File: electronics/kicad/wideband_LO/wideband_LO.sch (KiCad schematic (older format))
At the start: 25 parts, among them U1 BFP620

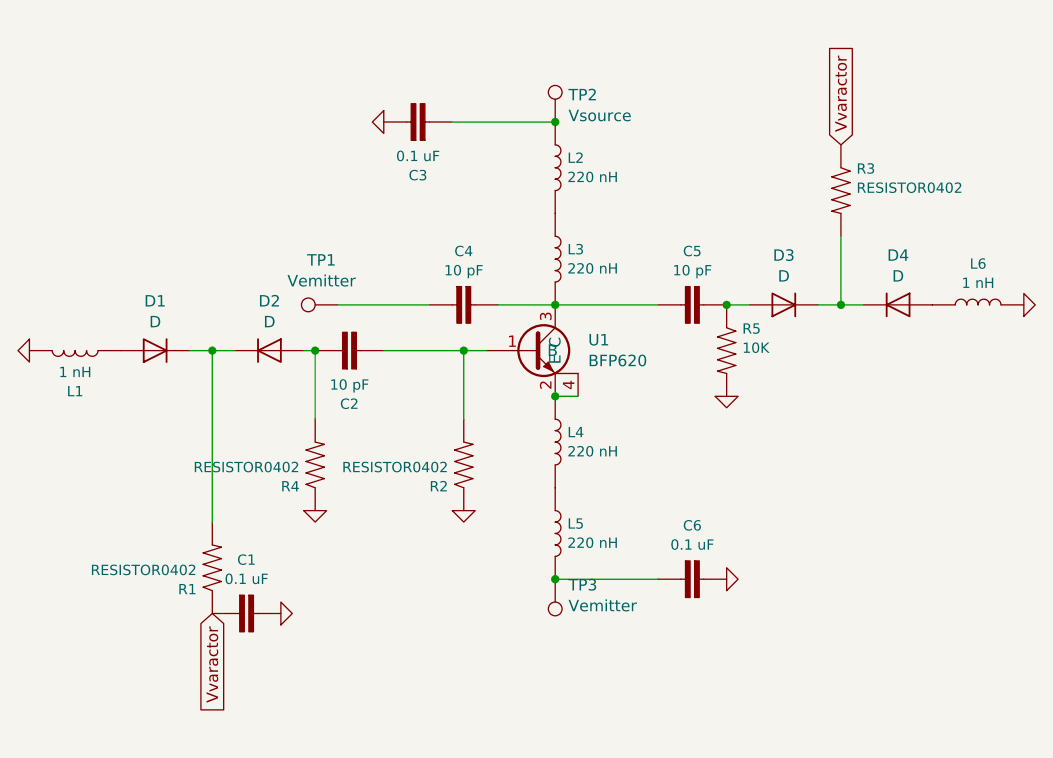
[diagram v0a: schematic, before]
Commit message: further fdtd
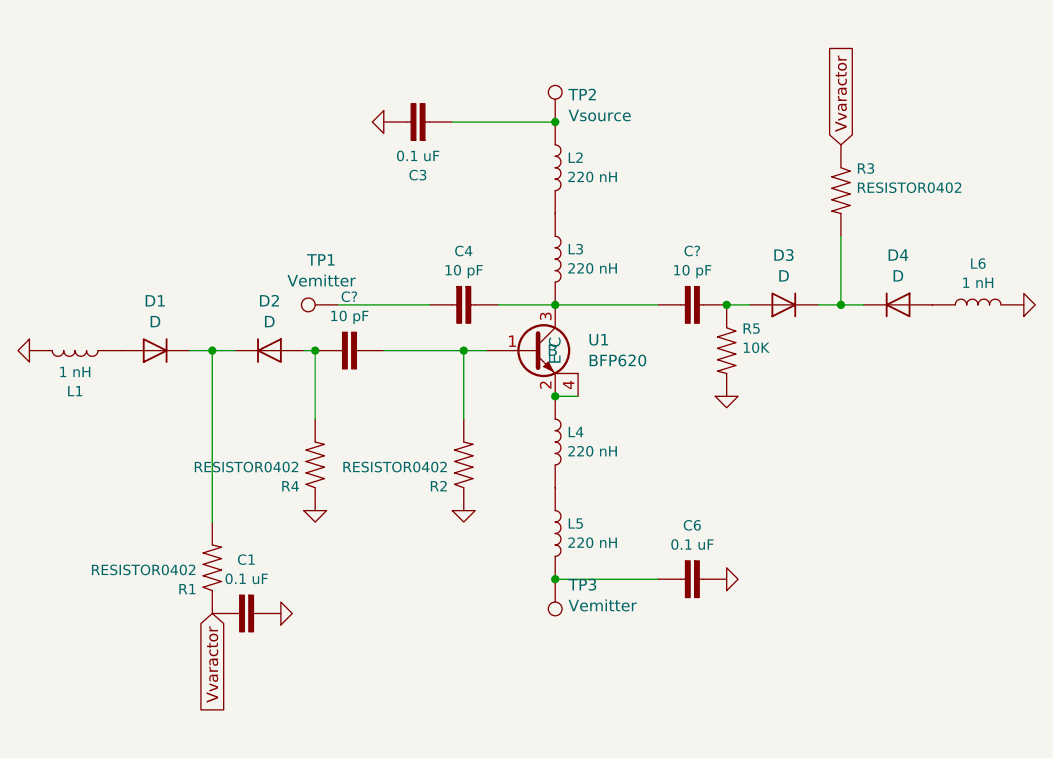
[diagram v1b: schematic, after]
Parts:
- removed C2, C5: 10 pF, 0402, symbol SparkFun-Capacitors:6PF-0402-50V-0.5%
- added C? (x2): 10 pF, 0402, symbol SparkFun-Capacitors:6PF-0402-50V-0.5%
- C4: Spice_Lib_File (none) -> /home/arthurdent/Projects/covidinator/electronics/models/10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; Spice_Model (none) -> 10pf0402; Spice_Netlist_Enabled (none) -> Y; Spice_Primitive (none) -> X
- D2: Spice_Lib_File (none) -> /home/arthurdent/Projects/covidinator/electronics/models/SM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; Spice_Model (none) -> SMV2019079LF; Spice_Netlist_Enabled (none) -> Y; Spice_Primitive (none) -> X
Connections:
- net at R2.2, U1.1 (B): now also C?.1
- net at C4.1, L3.2, U1.3 (C): now also C?.2
- net at D3.2 (A), R5.1: now also C?.1
- net at D2.2 (A), R4.2: now also C?.2
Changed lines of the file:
@@
 Wire Wire Line
 	3500 3050 3950 3050
-$Comp
-L SparkFun-Capacitors:6PF-0402-50V-0.5% C5
-U 1 1 5EE0CC0E
-P 4050 3050
-F 0 "C5" V 3816 3100 45  0000 C CNN
-F 1 "10 pF" V 3900 3100 45  0000 C CNN
-F 2 "0402" H 4050 3300 20  0001 C CNN
-F 3 "" H 4050 3050 50  0001 C CNN
-F 4 "" H 4158 3016 60  0000 L CNN "Field4"
-	1    4050 3050
-	0    1    1    0
-$EndComp
 Wire Wire Line
 	4850 3050 4750 3050
@@
 Wire Wire Line
 	3200 3250 3100 3250
-$Comp
-L SparkFun-Capacitors:6PF-0402-50V-0.5% C2
-U 1 1 5EE21BEE
-P 2650 3250
-F 0 "C2" V 2416 3300 45  0000 C CNN
-F 1 "10 pF" V 2500 3300 45  0000 C CNN
-F 2 "0402" H 2650 3500 20  0001 C CNN
-F 3 "" H 2650 3250 50  0001 C CNN
-F 4 "" H 2758 3216 60  0000 L CNN "Field4"
-	1    2650 3250
-	0    -1   -1   0
-$EndComp
 Wire Wire Line
 	1900 3250 2000 3250
-$Comp
-L SparkFun-Coils:INDUCTOR-0402-3.9NH L1
-U 1 1 5EE21BFD
-P 1400 3250
-F 0 "L1" V 1579 3250 45  0000 C CNN
-F 1 "1 nH" V 1495 3250 45  0000 C CNN
-F 2 "0402" H 1400 3500 20  0001 C CNN
-F 3 "" H 1400 3250 50  0001 C CNN
-F 4 "" H 1452 3166 60  0000 L CNN "Field4"
-	1    1400 3250
-	0    1    1    0
-$EndComp
-$Comp
-L power:GND #PWR0102
-U 1 1 5EE21C04
-P 1200 3250
-F 0 "#PWR0102" H 1200 3250 30  0001 C CNN
-F 1 "GND" H 1200 3180 30  0001 C CNN
-F 2 "" H 1200 3250 50  0001 C CNN
-F 3 "" H 1200 3250 50  0001 C CNN
-	1    1200 3250
-	0    1    1    0
-$EndComp
 $Comp
 L SparkFun-Resistors:RESISTOR0402 R1
@@
 F 3 "" H 3050 3050 50  0001 C CNN
 F 4 "" H 3158 3016 60  0000 L CNN "Field4"
+F 5 "X" H 3050 3050 50  0001 C CNN "Spice_Primitive"
+F 6 "10pf0402" H 3050 3050 50  0001 C CNN "Spice_Model"
+F 7 "Y" H 3050 3050 50  0001 C CNN "Spice_Netlist_Enabled"
+F 8 "/home/arthurdent/Projects/covidinator/electronics/models/10pf0402.lib" H 3050 3050 50  0001 C CNN "Spice_Lib_File"
 	1    3050 3050
 	0    1    1    0
@@
 F 2 "Diode_SMD:D_SOD-523" H 2250 3250 50  0001 C CNN
 F 3 "~" H 2250 3250 50  0001 C CNN
+F 4 "X" H 2250 3250 50  0001 C CNN "Spice_Primitive"
+F 5 "SMV2019079LF" H 2250 3250 50  0001 C CNN "Spice_Model"
+F 6 "Y" H 2250 3250 50  0001 C CNN "Spice_Netlist_Enabled"
+F 7 "/home/arthurdent/Projects/covidinator/electronics/models/SMV2019079LF.lib" H 2250 3250 50  0001 C CNN "Spice_Lib_File"
 	1    2250 3250
 	1    0    0    -1
@@
 Wire Wire Line
 	2400 3250 2450 3250
-Connection ~ 2450 3250
 $Comp
 L Device:D D3
@@
 Wire Wire Line
 	4350 3050 4250 3050
+$Comp
+L power:GND #PWR0102
+U 1 1 5EE21C04
+P 1200 3250
+F 0 "#PWR0102" H 1200 3250 30  0001 C CNN
+F 1 "GND" H 1200 3180 30  0001 C CNN
+F 2 "" H 1200 3250 50  0001 C CNN
+F 3 "" H 1200 3250 50  0001 C CNN
+	1    1200 3250
+	0    1    1    0
+$EndComp
+$Comp
+L SparkFun-Coils:INDUCTOR-0402-3.9NH L1
+U 1 1 5EE21BFD
+P 1400 3250
+F 0 "L1" V 1579 3250 45  0000 C CNN
+F 1 "1 nH" V 1495 3250 45  0000 C CNN
+F 2 "0402" H 1400 3500 20  0001 C CNN
+F 3 "" H 1400 3250 50  0001 C CNN
+F 4 "" H 1452 3166 60  0000 L CNN "Field4"
+	1    1400 3250
+	0    1    1    0
+$EndComp
+$Comp
+L SparkFun-Capacitors:6PF-0402-50V-0.5% C?
+U 1 1 5EEB34DA
+P 4050 3050
+F 0 "C?" V 3816 3100 45  0000 C CNN
+F 1 "10 pF" V 3900 3100 45  0000 C CNN
+F 2 "0402" H 4050 3300 20  0001 C CNN
+F 3 "" H 4050 3050 50  0001 C CNN
+F 4 "" H 4158 3016 60  0000 L CNN "Field4"
+F 5 "X" H 4050 3050 50  0001 C CNN "Spice_Primitive"
+F 6 "10pf0402" H 4050 3050 50  0001 C CNN "Spice_Model"
+F 7 "Y" H 4050 3050 50  0001 C CNN "Spice_Netlist_Enabled"
+F 8 "/home/arthurdent/Projects/covidinator/electronics/models/10pf0402.lib" H 4050 3050 50  0001 C CNN "Spice_Lib_File"
+	1    4050 3050
+	0    1    1    0
+$EndComp
 Connection ~ 4250 3050
+$Comp
+L SparkFun-Capacitors:6PF-0402-50V-0.5% C?
+U 1 1 5EEB3D3A
+P 2550 3250
+F 0 "C?" V 2316 3300 45  0000 C CNN
+F 1 "10 pF" V 2400 3300 45  0000 C CNN
+F 2 "0402" H 2550 3500 20  0001 C CNN
+F 3 "" H 2550 3250 50  0001 C CNN
+F 4 "" H 2658 3216 60  0000 L CNN "Field4"
+F 5 "X" H 2550 3250 50  0001 C CNN "Spice_Primitive"
+F 6 "10pf0402" H 2550 3250 50  0001 C CNN "Spice_Model"
+F 7 "Y" H 2550 3250 50  0001 C CNN "Spice_Netlist_Enabled"
+F 8 "/home/arthurdent/Projects/covidinator/electronics/models/10pf0402.lib" H 2550 3250 50  0001 C CNN "Spice_Lib_File"
+	1    2550 3250
+	0    1    1    0
+$EndComp
+Connection ~ 2450 3250
 $EndSCHEMATC
